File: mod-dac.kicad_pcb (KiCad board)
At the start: 2 copper layers, 62 parts, among them J1 digi in, J2 cv out, P1 MTA-156-4, U1 TL074, U2 TL074, U4 DAC8168, U5 LD2981

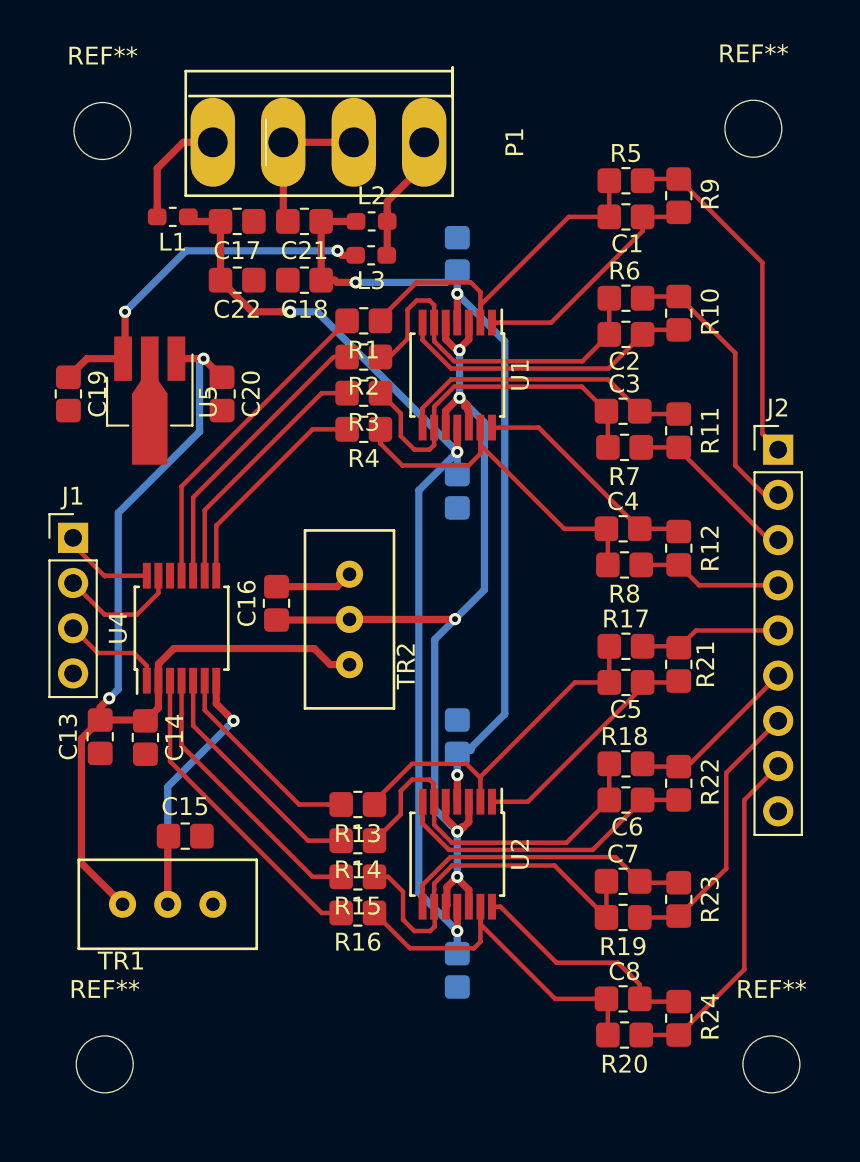
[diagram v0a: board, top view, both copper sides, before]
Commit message: edge cut
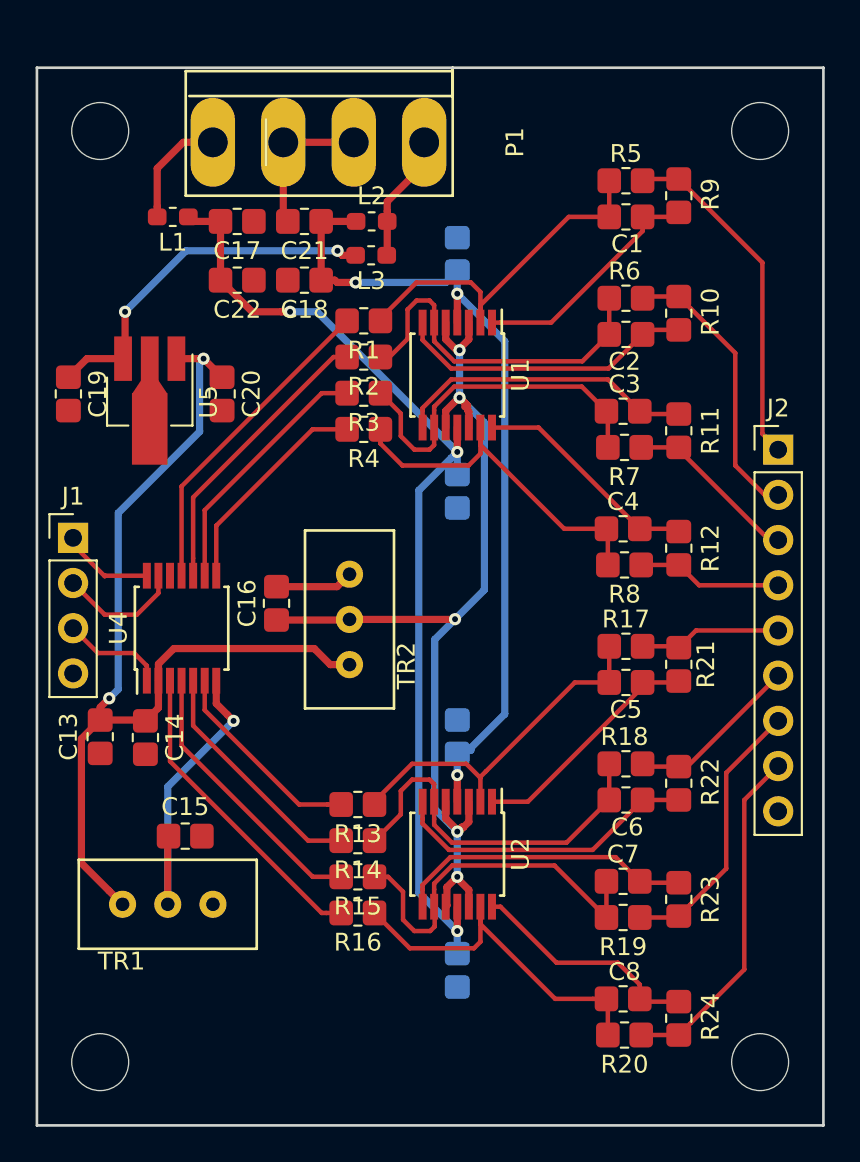
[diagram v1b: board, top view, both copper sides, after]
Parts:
- removed REF**: MountingHole_3.2mm_M3, MountingHole:MountingHole_3.2mm_M3
- added REF1: MountingHole_3.2mm_M3, MountingHole:MountingHole_3.2mm_M3, F.Cu at (85.9, 58.9)
- moved REF4 0.65 mm to (122.9, 111.3)
- moved REF2 0.40 mm to (122.9, 58.9)
- moved REF3 0.28 mm to (85.9, 111.3)
- renumbered REF** to REF2, REF** to REF3, REF** to REF4
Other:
- board outline added: 44.2 x 59.4 mm
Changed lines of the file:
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@@
   (general
     (thickness 1.6)
-    (drawings 0)
+    (drawings 1)
     (tracks 364)
     (zones 0)
@@
   )
   (module MountingHole:MountingHole_3.2mm_M3 (layer F.Cu)
-    (at 122.555 58.801)
+    (at 122.936 58.928)
     (descr "Mounting Hole 3.2mm, no annular, M3")
     (tags "mounting hole 3.2mm no annular m3")
     (attr virtual)
-    (fp_text reference REF** (at 0 -4.2) (layer F.SilkS)
+    (fp_text reference REF2 (at 0 -4.2) (layer F.Fab) hide
       (effects (font (size 1 1) (thickness 0.15)))
     )
@@
   )
   (module MountingHole:MountingHole_3.2mm_M3 (layer F.Cu)
-    (at 123.571 111.379)
+    (at 122.936 111.252)
     (descr "Mounting Hole 3.2mm, no annular, M3")
     (tags "mounting hole 3.2mm no annular m3")
     (attr virtual)
-    (fp_text reference REF** (at 0 -4.2) (layer F.SilkS)
+    (fp_text reference REF4 (at 0 -4.2) (layer F.Fab) hide
       (effects (font (size 1 1) (thickness 0.15)))
     )
@@
   )
   (module MountingHole:MountingHole_3.2mm_M3 (layer F.Cu)
-    (at 86.106 111.379)
+    (at 85.852 111.252)
     (descr "Mounting Hole 3.2mm, no annular, M3")
     (tags "mounting hole 3.2mm no annular m3")
     (attr virtual)
-    (fp_text reference REF** (at 0 -4.2) (layer F.SilkS)
+    (fp_text reference REF3 (at 0 -4.2) (layer F.Fab) hide
       (effects (font (size 1 1) (thickness 0.15)))
     )
@@
   )
   (module MountingHole:MountingHole_3.2mm_M3 (layer F.Cu)
-    (at 85.979 58.928)
+    (at 85.852 58.928)
     (descr "Mounting Hole 3.2mm, no annular, M3")
     (tags "mounting hole 3.2mm no annular m3")
     (attr virtual)
-    (fp_text reference REF** (at 0 -4.2) (layer F.SilkS)
+    (fp_text reference REF1 (at 0 -4.2) (layer F.Fab) hide
       (effects (font (size 1 1) (thickness 0.15)))
     )
@@
     (pad 1 np_thru_hole circle (at 0 0) (size 3.2 3.2) (drill 3.2) (layers *.Cu *.Mask))
   )
+  (gr_poly (pts (xy 82.296 55.372) (xy 126.492 55.372) (xy 126.492 114.808) (xy 82.296 114.808)) (layer Edge.Cuts) (width 0.15))
   (segment (start 114.457 61.722) (end 114.457 63.754) (width 0.254) (layer F.Cu) (net 1))
   (segment (start 112.179 63.754) (end 107.218 68.715) (width 0.254) (layer F.Cu) (net 1))
